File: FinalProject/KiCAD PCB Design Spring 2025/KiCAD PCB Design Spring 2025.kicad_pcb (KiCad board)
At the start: 2 copper layers, 17 parts, among them J1 Motor_Servo, J2 Ultrasonic HS-SR04, M1 Motor_DC, U1 ATmega328PB-A, U2 74HC595, U3 BMI160, U4 CA56-12EWA, U5 74HC595, U6 ROB-14450

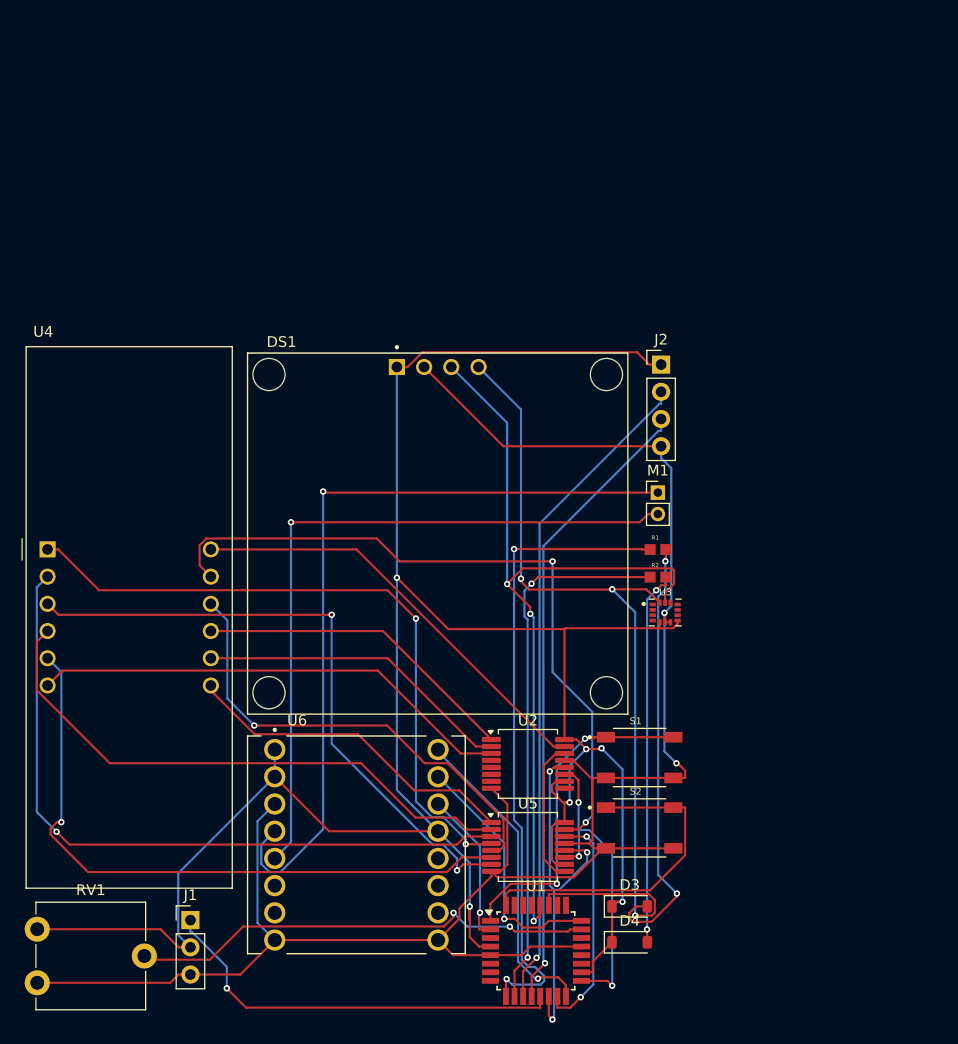
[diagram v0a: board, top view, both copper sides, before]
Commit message: KiCAD PCB Design Spring 2025
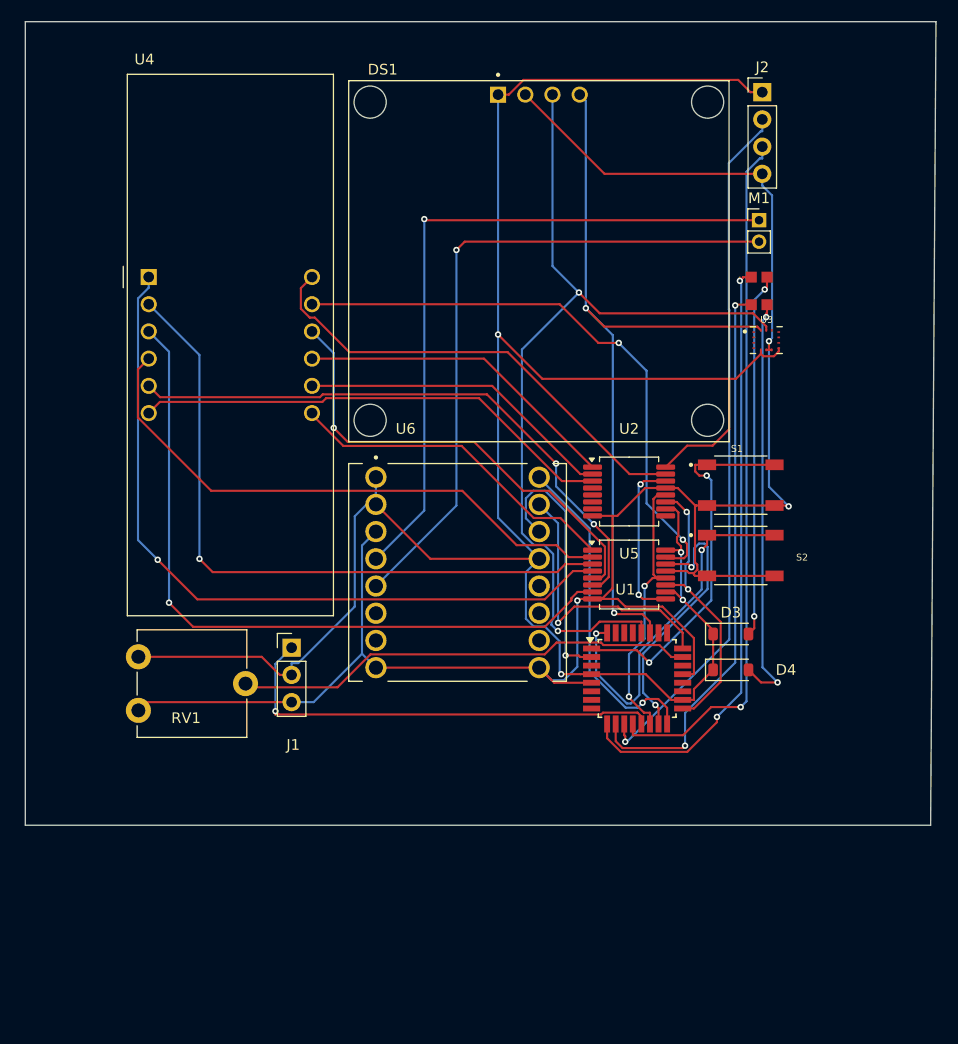
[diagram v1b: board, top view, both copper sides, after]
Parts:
- moved RV1 27.1 mm to (111.1, 103.8)
- moved U2 27.1 mm to (156.9, 83.3)
- moved U5 27.1 mm to (156.9, 91.1)
- moved M1 27.1 mm to (169.0, 58.0)
- moved DS1 27.1 mm to (148.4, 61.9)
- moved R1 27.1 mm to (169.0, 63.3)
- moved J1 27.1 mm to (125.4, 97.9)
- moved D3 27.1 mm to (166.3, 96.7)
- moved D4 27.1 mm to (166.3, 100.0)
- moved J2 27.1 mm to (169.3, 46.1)
- moved R2 27.1 mm to (169.0, 65.9)
- moved S1 27.1 mm to (167.3, 82.8)
- moved S2 27.1 mm to (167.3, 89.3)
- moved U1 27.1 mm to (157.6, 100.8)
- moved U3 27.1 mm to (169.7, 69.2)
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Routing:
- net Net-(U4-a): track 65.9 -> 54.7 mm
- net SDA: track 82.1 -> 71.6 mm, vias 3 -> 2
- net Net-(U1-PD4): track 14.4 -> 24.4 mm
- net VCC: track 229.1 -> 219.3 mm, vias 6 -> 4
- net Net-(M1-+): track 74.1 -> 64.9 mm
- net Latch: track 34.5 -> 25.7 mm, vias 3 -> 2
- net Net-(U4-DPX): track 59.7 -> 68.0 mm, vias 2 -> 1
- net Net-(U4-e): track 63.1 -> 70.8 mm, vias 2 -> 1
- net SCL: track 76.4 -> 83.8 mm, vias 3 -> 2
- net Net-(D3-A): track 41.4 -> 34.0 mm
- net Echo: track 59.1 -> 65.5 mm
- net Net-(U4-g): track 60.8 -> 55.7 mm, vias 1 -> 2
- net GND: track 184.7 -> 189.7 mm, vias 2 -> 3
- net Net-(D4-A): track 35.1 -> 39.2 mm
- net MOSI: track 21.4 -> 25.6 mm
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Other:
- board outline added: 85 x 75 mm
